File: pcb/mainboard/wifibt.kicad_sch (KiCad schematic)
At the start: 10 parts

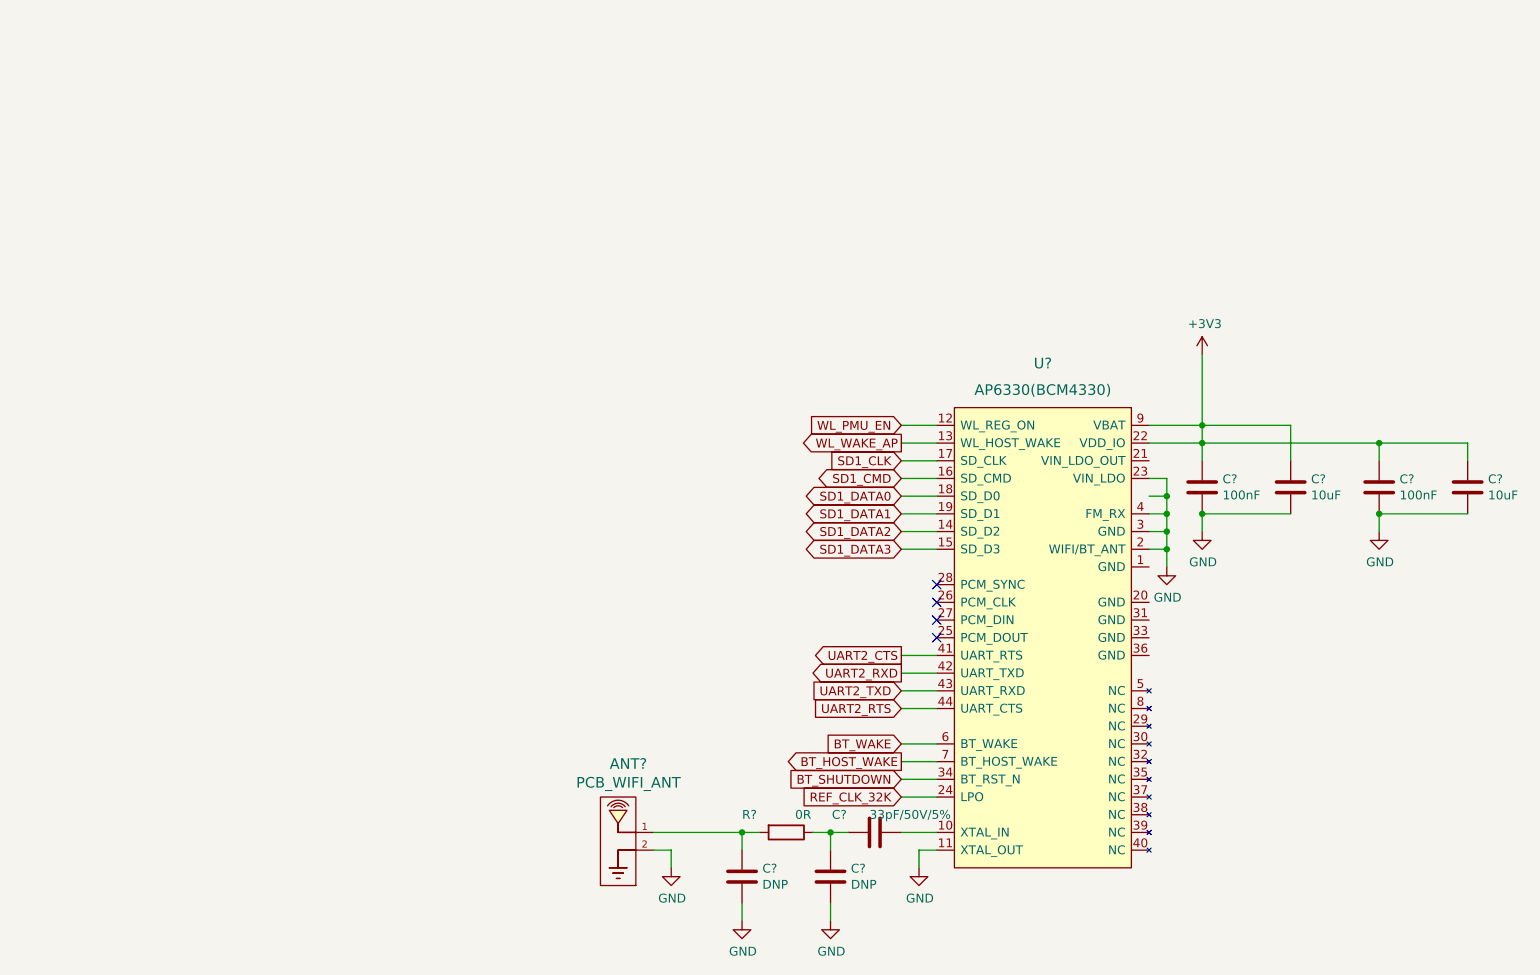
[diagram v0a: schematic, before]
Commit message: Working on mainboard schematics
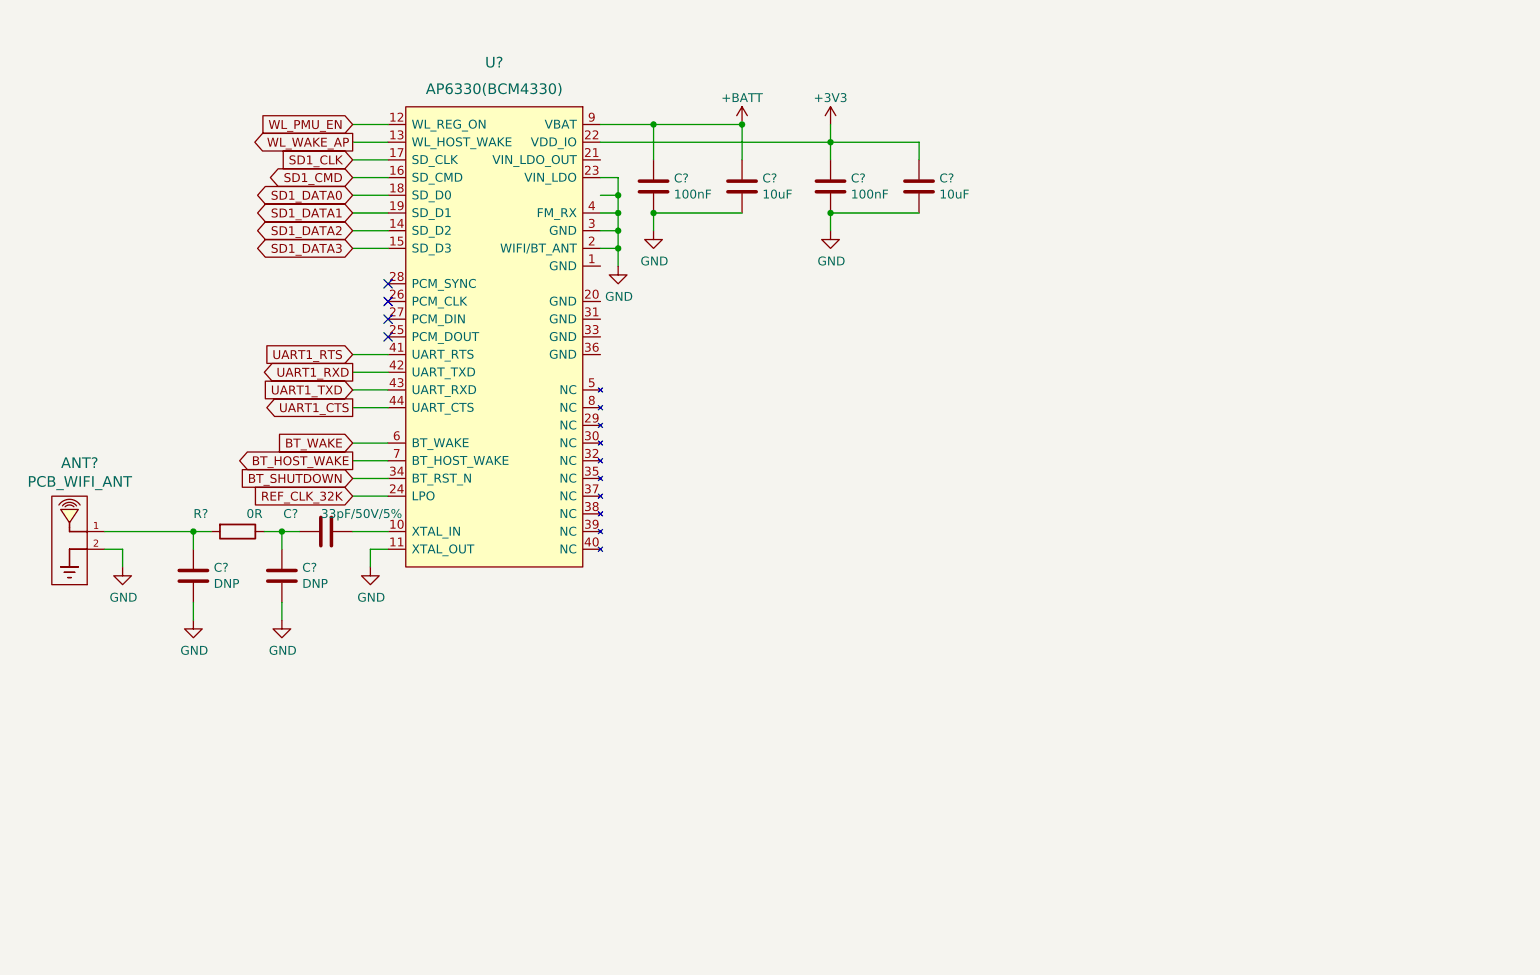
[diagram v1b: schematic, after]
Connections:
- net +3V3: no longer C?.1, C?.1, U?.9 (VBAT)
- net UART2_CTS renamed UART1_RTS
- net UART2_RTS renamed UART1_CTS
- net UART2_RXD renamed UART1_RXD
- net UART2_TXD renamed UART1_TXD
- new net +BATT: C?.1, C?.1, U?.9 (VBAT)
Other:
- moved on the sheet: ANT?, C?, R?, U?

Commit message: Mainboard schematics WIP
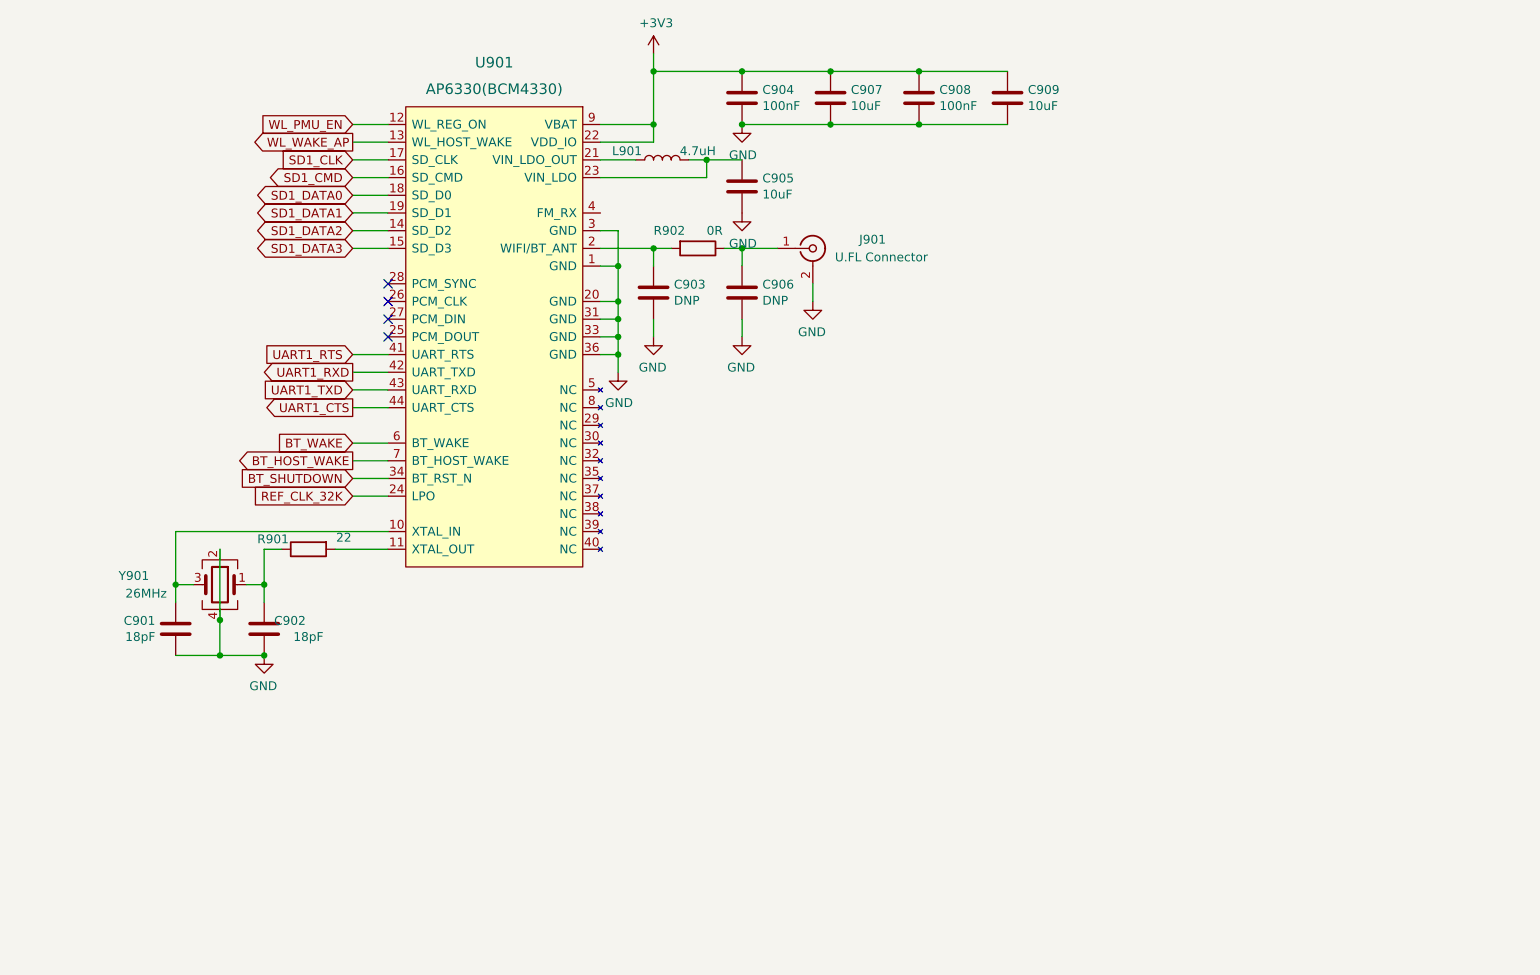
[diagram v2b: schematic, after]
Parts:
- removed ANT?: PCB_WIFI_ANT, footprints:bt_antenna_1ant_2gnd, symbol symbols:WIFI_ANT_ESP8266
- removed C?: 33pF/50V/5%, Capacitor_SMD:C_0402_1005Metric, symbol Device:C
- removed C? (x2): 100nF, Capacitor_SMD:C_0402_1005Metric, symbol Device:C
- removed C? (x2): 10uF, Capacitor_SMD:C_0603_1608Metric, symbol Device:C
- removed C? (x2): DNP, Capacitor_SMD:C_0402_1005Metric, symbol Device:C
- removed R?: 0R, Resistor_SMD:R_0402_1005Metric, symbol Device:R
- added C901, C902: 18pF, Capacitor_SMD:C_0402_1005Metric, symbol Device:C
- added C903, C906: DNP, Capacitor_SMD:C_0402_1005Metric, symbol Device:C
- added C904, C908: 100nF, Capacitor_SMD:C_0402_1005Metric, symbol Device:C
- added C905, C907, C909: 10uF, Capacitor_SMD:C_0603_1608Metric, symbol Device:C
- added J901: U.FL Connector, Connector_Coaxial:U.FL_Molex_MCRF_73412-0110_Vertical, symbol Connector:Conn_Coaxial
- added L901: 4.7uH, footprints:L_1212, symbol Device:L
- added R901: 22, Resistor_SMD:R_0402_1005Metric, symbol Device:R
- added R902: 0R, Resistor_SMD:R_0402_1005Metric, symbol Device:R
- added Y901: 26MHz, Oscillator:Oscillator_SMD_Abracon_ASE-4Pin_3.2x2.5mm, symbol Device:Crystal_GND24
- gave numbers to parts that had none: 1
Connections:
- net +BATT is gone; now on net +3V3: U901.9 (VBAT)
- net +3V3: now also C904.1, C907.1, C908.1, C909.1
- net GND: now also U901.1 (GND), U901.20 (GND), U901.31 (GND), U901.33 (GND), U901.36 (GND), C901.2, C902.2, C903.1, C904.2, C905.2, C906.1, C907.2, C908.2, C909.2, J901.2 (Ext), Y901.2, Y901.4; no longer U901.11 (XTAL_OUT), U901.2 (WIFI/BT_ANT), U901.23 (VIN_LDO), U901.4 (FM_RX)
- net at U901.10 (XTAL_IN): now also C901.1, Y901.3
- net at U901.21 (VIN_LDO_OUT): now also L901.1
- new net: C902.1, R901.1, Y901.1
- new net: C905.1, L901.2, U901.23 (VIN_LDO)
- new net: C903.2, R902.2, U901.2 (WIFI/BT_ANT)
- new net: C906.2, J901.1 (In), R902.1
- new net: R901.2, U901.11 (XTAL_OUT)
